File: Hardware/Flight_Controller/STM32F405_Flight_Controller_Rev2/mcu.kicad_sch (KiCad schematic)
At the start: 18 parts, among them U1 STM32F405RGTx, Y1 Crystal

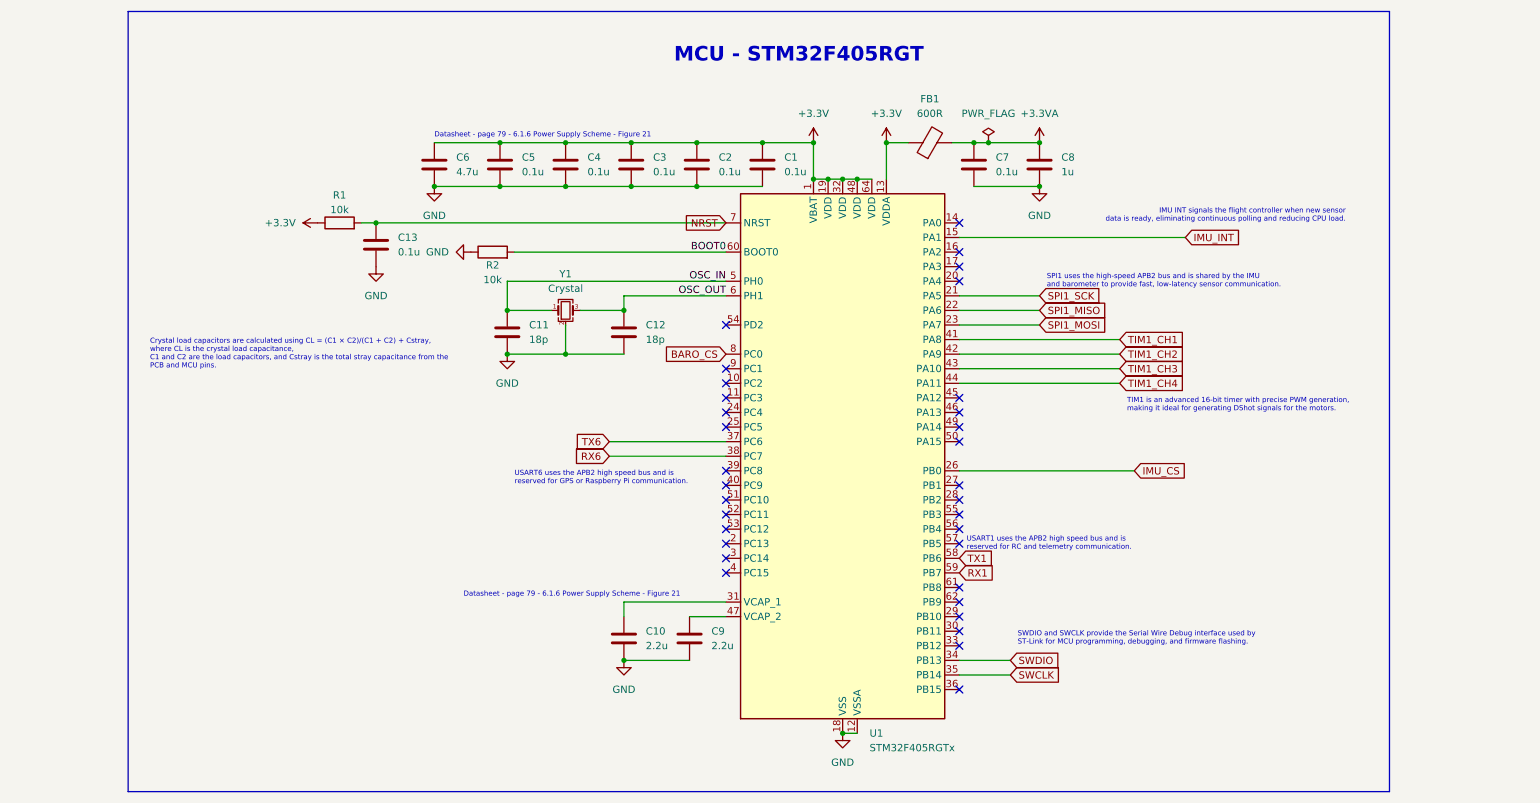
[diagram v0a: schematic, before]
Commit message: Ready Rev2 PCB
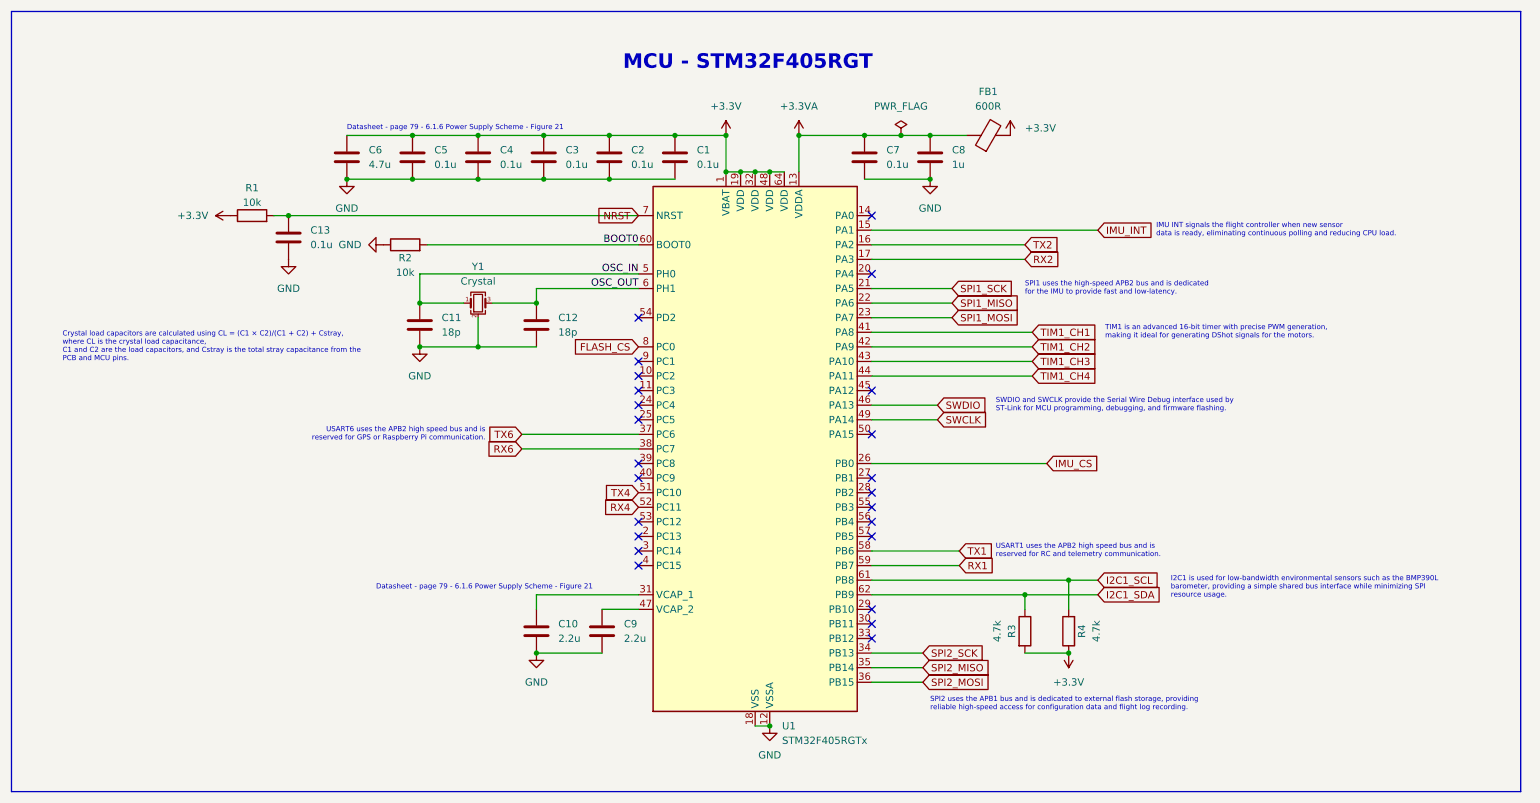
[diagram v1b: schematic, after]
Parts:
- added R3, R4: 4.7k, Resistor_SMD:R_0603_1608Metric_Pad0.98x0.95mm_HandSolder, symbol Device:R
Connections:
- net +3.3V: now also FB1.2, R3.2, R4.1; no longer FB1.1, U1.13 (VDDA)
- net +3.3VA: now also FB1.1, U1.13 (VDDA); no longer FB1.2
- net SWCLK: now also U1.49 (PA14); no longer U1.35 (PB14)
- net SWDIO: now also U1.46 (PA13); no longer U1.34 (PB13)
- net TX2: now reaches U1.16 (PA2)
- net RX2: now reaches U1.17 (PA3)
- net SPI2_MOSI: now reaches U1.36 (PB15)
- net TX4: now reaches U1.51 (PC10)
- net RX4: now reaches U1.52 (PC11)
- net I2C1_SCL: now reaches U1.61 (PB8)
- net I2C1_SCL: now also R4.2
- net I2C1_SDA: now reaches U1.62 (PB9)
- net I2C1_SDA: now also R3.1
- net BARO_CS renamed FLASH_CS
- new net SPI2_MISO: U1.35 (PB14)
- new net SPI2_SCK: U1.34 (PB13)
- no-connect marks 33 -> 24
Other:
- note added: "I2C1 is used for low-bandwidth environmental sensors such as the BMP390L barometer, providing a simple shared bus interface while minimizing SPI resource usage."
- note added: "SPI1 uses the high-speed APB2 bus and is dedicated for the IMU to provide fast and low-latency."
- note added: "SPI2 uses the APB1 bus and is dedicated to external flash storage, providing reliable high-speed access for configuration data and flight log recording."
- note removed: "SPI1 uses the high-speed APB2 bus and is shared by the IMU and barometer to provide fast, low-latency sensor communication."
- moved on the sheet: C1, C10, C11, C12, C13, C2, C3, C4, C5, C6, C7, C8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
